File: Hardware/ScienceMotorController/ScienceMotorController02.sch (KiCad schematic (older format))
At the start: 1 part, among them U1 TM4C129E_Launchpad

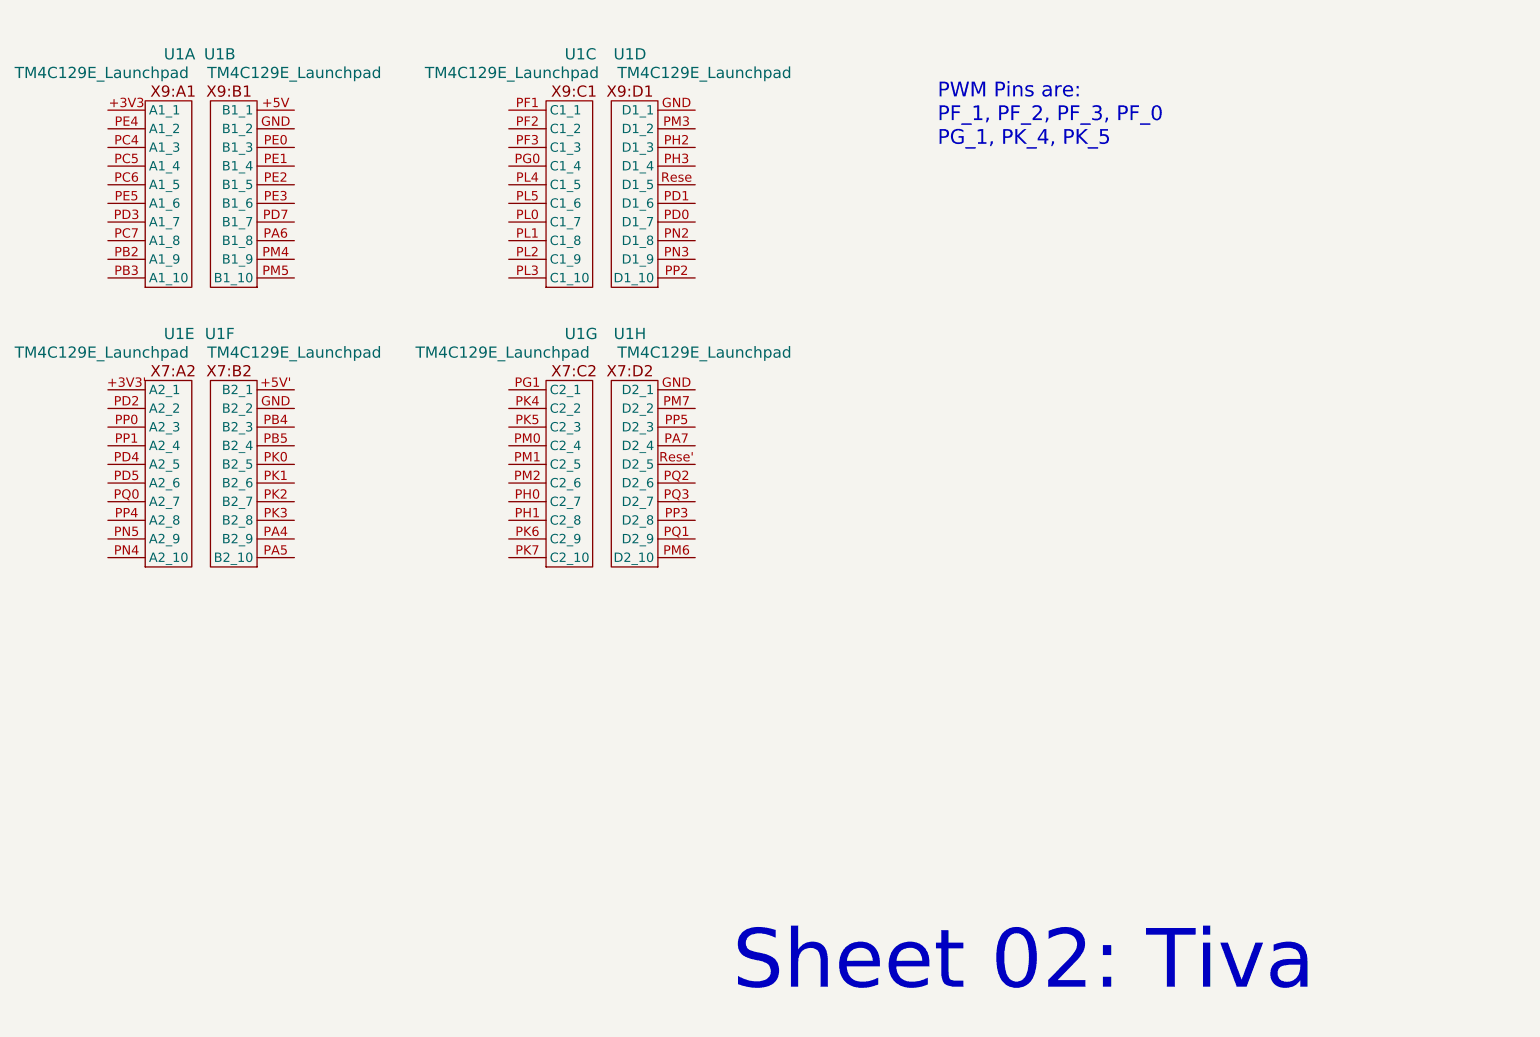
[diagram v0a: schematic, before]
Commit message: Flagged Tiva
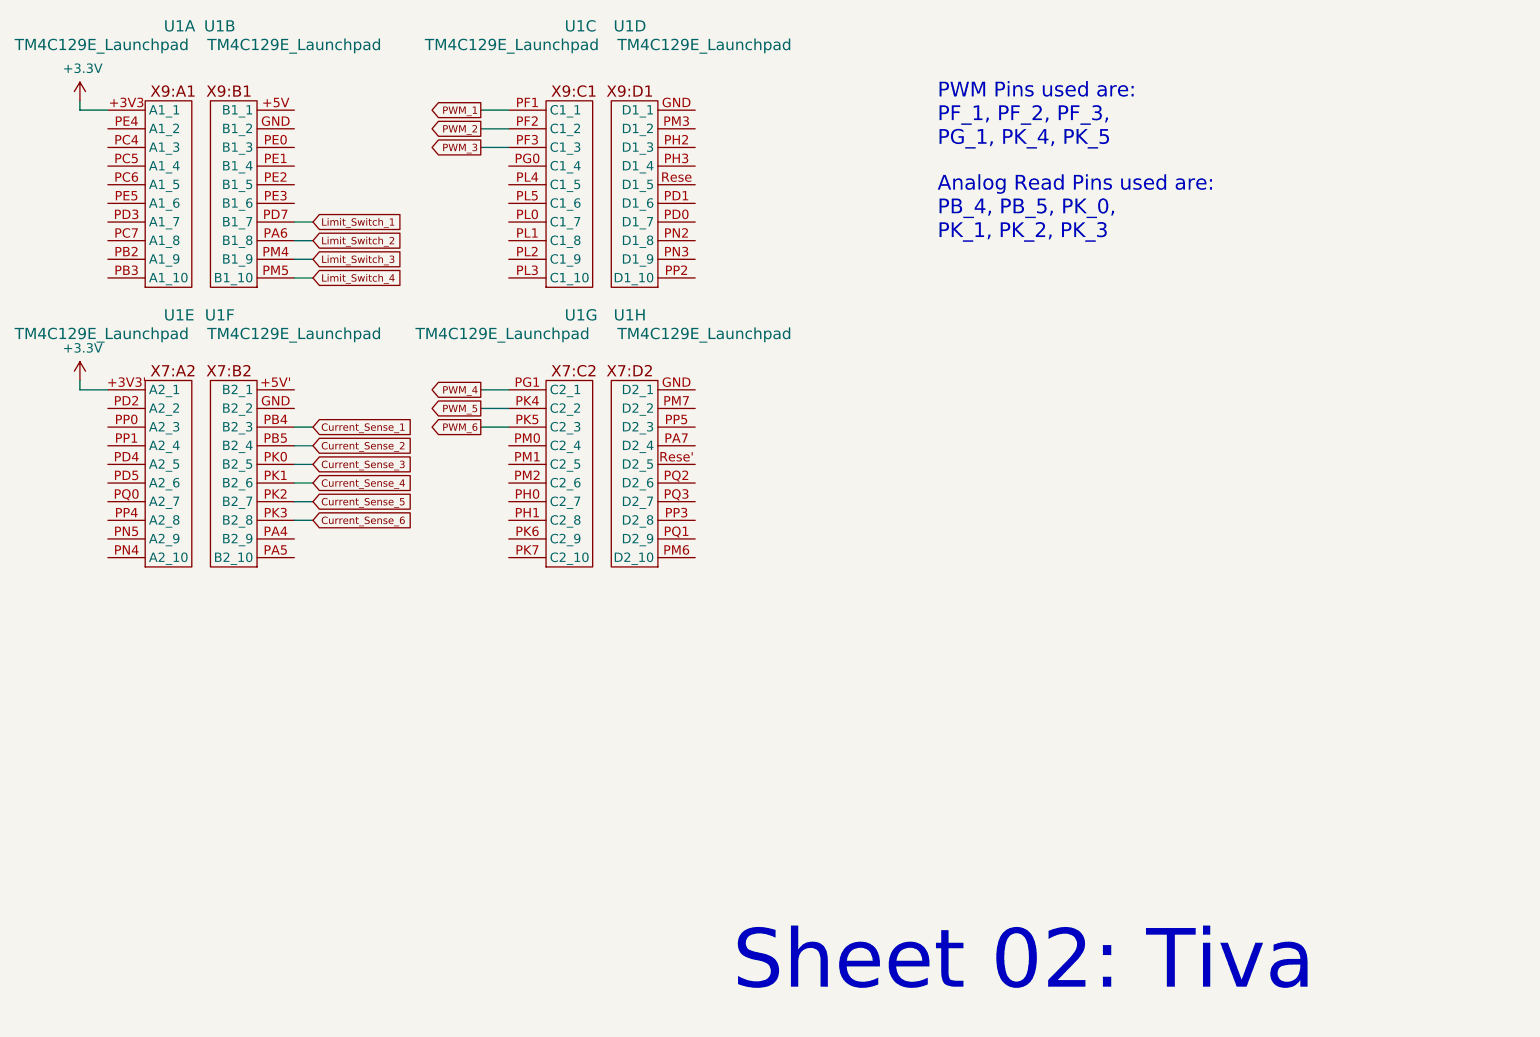
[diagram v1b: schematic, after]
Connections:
- net +3V3: now reaches U1.+3V3 (A1_1)
- net +3V3: now also U1.+3V3' (A2_1)
- net Limit_Switch_2: now reaches U1.PA6 (B1_8)
- net Limit_Switch_1: now reaches U1.PD7 (B1_7)
- net Limit_Switch_3: now reaches U1.PM4 (B1_9)
- net Limit_Switch_4: now reaches U1.PM5 (B1_10)
- net PWM_1: now reaches U1.PF1 (C1_1)
- net PWM_2: now reaches U1.PF2 (C1_2)
- net PWM_3: now reaches U1.PF3 (C1_3)
- net Current_Sense_1: now reaches U1.PB4 (B2_3)
- net Current_Sense_2: now reaches U1.PB5 (B2_4)
- net Current_Sense_3: now reaches U1.PK0 (B2_5)
- net Current_Sense_4: now reaches U1.PK1 (B2_6)
- net Current_Sense_5: now reaches U1.PK2 (B2_7)
- net Current_Sense_6: now reaches U1.PK3 (B2_8)
- net PWM_4: now reaches U1.PG1 (C2_1)
- net PWM_5: now reaches U1.PK4 (C2_2)
- net PWM_6: now reaches U1.PK5 (C2_3)
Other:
- note added: "Analog Read Pins used are:\nPB_4, PB_5, PK_0, \nPK_1, PK_2, PK_3"
- note added: "PWM Pins used are:\nPF_1, PF_2, PF_3, \nPG_1, PK_4, PK_5"
- note removed: "PWM Pins are:\nPF_1, PF_2, PF_3, PF_0\nPG_1, PK_4, PK_5"
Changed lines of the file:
@@
 U 1 1 5F715123
 P 4200 3200
-F 0 "U1" H 4300 4450 60  0000 L CNN
-F 1 "TM4C129E_Launchpad" H 3500 4350 60  0000 L CNN
+F 0 "U1" H 4300 4600 60  0000 L CNN
+F 1 "TM4C129E_Launchpad" H 3500 4500 60  0000 L CNN
 F 2 "" H 4200 3200 60  0001 C CNN
 F 3 "" H 4200 3200 60  0001 C CNN
@@
 U 2 1 5F716DA0
 P 4800 3200
-F 0 "U1" H 5000 4450 60  0000 C CNN
-F 1 "TM4C129E_Launchpad" H 4600 4350 60  0000 C CNN
+F 0 "U1" H 5000 4600 60  0000 C CNN
+F 1 "TM4C129E_Launchpad" H 4600 4500 60  0000 C CNN
 F 2 "" H 4800 3200 60  0001 C CNN
 F 3 "" H 4800 3200 60  0001 C CNN
@@
 U 3 1 5F7264AA
 P 6350 3200
-F 0 "U1" H 6450 4450 60  0000 L CNN
-F 1 "TM4C129E_Launchpad" H 5700 4350 60  0000 L CNN
+F 0 "U1" H 6450 4600 60  0000 L CNN
+F 1 "TM4C129E_Launchpad" H 5700 4500 60  0000 L CNN
 F 2 "" H 6350 3200 60  0001 C CNN
 F 3 "" H 6350 3200 60  0001 C CNN
@@
 U 4 1 5F72B226
 P 6950 3200
-F 0 "U1" H 7100 4450 60  0000 C CNN
-F 1 "TM4C129E_Launchpad" H 6700 4350 60  0000 C CNN
+F 0 "U1" H 7100 4600 60  0000 C CNN
+F 1 "TM4C129E_Launchpad" H 6700 4500 60  0000 C CNN
 F 2 "" H 6950 3200 60  0001 C CNN
 F 3 "" H 6950 3200 60  0001 C CNN
@@
 U 5 1 5F733DC7
 P 4200 4700
-F 0 "U1" H 4300 5950 60  0000 L CNN
-F 1 "TM4C129E_Launchpad" H 3500 5850 60  0000 L CNN
+F 0 "U1" H 4300 6050 60  0000 L CNN
+F 1 "TM4C129E_Launchpad" H 3500 5950 60  0000 L CNN
 F 2 "" H 4200 4700 60  0001 C CNN
 F 3 "" H 4200 4700 60  0001 C CNN
@@
 U 6 1 5F73B2DD
 P 4800 4700
-F 0 "U1" H 5000 5950 60  0000 C CNN
-F 1 "TM4C129E_Launchpad" H 4600 5850 60  0000 C CNN
+F 0 "U1" H 5000 6050 60  0000 C CNN
+F 1 "TM4C129E_Launchpad" H 4600 5950 60  0000 C CNN
 F 2 "" H 4800 4700 60  0001 C CNN
 F 3 "" H 4800 4700 60  0001 C CNN
@@
 U 7 1 5F740CF4
 P 6350 4700
-F 0 "U1" H 6450 5950 60  0000 L CNN
-F 1 "TM4C129E_Launchpad" H 5650 5850 60  0000 L CNN
+F 0 "U1" H 6450 6050 60  0000 L CNN
+F 1 "TM4C129E_Launchpad" H 5650 5950 60  0000 L CNN
 F 2 "" H 6350 4700 60  0001 C CNN
 F 3 "" H 6350 4700 60  0001 C CNN
@@
 U 8 1 5F7529E8
 P 6950 4700
-F 0 "U1" H 7100 5950 60  0000 C CNN
-F 1 "TM4C129E_Launchpad" H 6700 5850 60  0000 C CNN
+F 0 "U1" H 7100 6050 60  0000 C CNN
+F 1 "TM4C129E_Launchpad" H 6700 5950 60  0000 C CNN
 F 2 "" H 6950 4700 60  0001 C CNN
 F 3 "" H 6950 4700 60  0001 C CNN
@@
 $EndComp
 Text Notes 8450 2450 0    79   ~ 0
-PWM Pins are:\nPF_1, PF_2, PF_3, PF_0\nPG_1, PK_4, PK_5
+PWM Pins used are:\nPF_1, PF_2, PF_3, \nPG_1, PK_4, PK_5
+Text GLabel 6000 2250 0    39   Output ~ 0
+PWM_1
+Wire Wire Line
+	6000 2250 6150 2250
+Text GLabel 6000 2350 0    39   Output ~ 0
+PWM_2
+Wire Wire Line
+	6150 2350 6000 2350
+Text GLabel 6000 2450 0    39   Output ~ 0
+PWM_3
+Wire Wire Line
+	6000 2450 6150 2450
+Wire Wire Line
+	4000 2250 3850 2250
+Wire Wire Line
+	3850 2250 3850 2200
+$Comp
+L power:+3.3V #PWR?
+U 1 1 5FB06302
+P 3850 2200
+F 0 "#PWR?" H 3850 2050 50  0001 C CNN
+F 1 "+3.3V" H 3865 2373 50  0000 C CNN
+F 2 "" H 3850 2200 50  0001 C CNN
+F 3 "" H 3850 2200 50  0001 C CNN
+	1    3850 2200
+	1    0    0    -1
+$EndComp
+Text GLabel 6000 3750 0    39   Output ~ 0
+PWM_4
+Text GLabel 6000 3850 0    39   Output ~ 0
+PWM_5
+Text GLabel 6000 3950 0    39   Output ~ 0
+PWM_6
+Wire Wire Line
+	6000 3750 6150 3750
+Wire Wire Line
+	6150 3850 6000 3850
+Wire Wire Line
+	6150 3950 6000 3950
+Text Notes 8450 2950 0    79   ~ 0
+Analog Read Pins used are:\nPB_4, PB_5, PK_0, \nPK_1, PK_2, PK_3
+Text GLabel 5100 3950 2    39   Input ~ 0
+Current_Sense_1
+Wire Wire Line
+	5100 3950 5000 3950
+Wire Wire Line
+	5000 4050 5100 4050
+Wire Wire Line
+	5000 4150 5100 4150
+Wire Wire Line
+	5000 4250 5100 4250
+Wire Wire Line
+	5000 4350 5100 4350
+Wire Wire Line
+	5000 4450 5100 4450
+Text GLabel 5100 4050 2    39   Input ~ 0
+Current_Sense_2
+Text GLabel 5100 4150 2    39   Input ~ 0
+Current_Sense_3
+Text GLabel 5100 4250 2    39   Input ~ 0
+Current_Sense_4
+Text GLabel 5100 4350 2    39   Input ~ 0
+Current_Sense_5
+Text GLabel 5100 4450 2    39   Input ~ 0
+Current_Sense_6
+$Comp
+L power:+3.3V #PWR?
+U 1 1 5FB0EFA7
+P 3850 3700
+F 0 "#PWR?" H 3850 3550 50  0001 C CNN
+F 1 "+3.3V" H 3865 3873 50  0000 C CNN
+F 2 "" H 3850 3700 50  0001 C CNN
+F 3 "" H 3850 3700 50  0001 C CNN
+	1    3850 3700
+	1    0    0    -1
+$EndComp
+Wire Wire Line
+	3850 3700 3850 3750
+Wire Wire Line
+	3850 3750 4000 3750
+Text GLabel 5100 2850 2    39   Input ~ 0
+Limit_Switch_1
+Wire Wire Line
+	5100 2850 5000 2850
+Text GLabel 5100 2950 2    39   Input ~ 0
+Limit_Switch_2
+Text GLabel 5100 3050 2    39   Input ~ 0
+Limit_Switch_3
+Text GLabel 5100 3150 2    39   Input ~ 0
+Limit_Switch_4
+Wire Wire Line
+	5100 2950 5000 2950
+Wire Wire Line
+	5000 3050 5100 3050
+Wire Wire Line
+	5100 3150 5000 3150
 Text Notes 7350 7000 0    315  ~ 0
 Sheet 02: Tiva
